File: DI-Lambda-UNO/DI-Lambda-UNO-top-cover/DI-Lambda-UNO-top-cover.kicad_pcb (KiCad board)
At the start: 2 copper layers, 38.2 x 68.5 mm, 7 parts, among them J12 Conn_01x05, J13 Conn_01x11, J5 Conn_01x11, SW2 SW_BLANK, SW3 SW_SAMPLE, SW4 SW_MODE, U1 LCD_1.44_ST7735

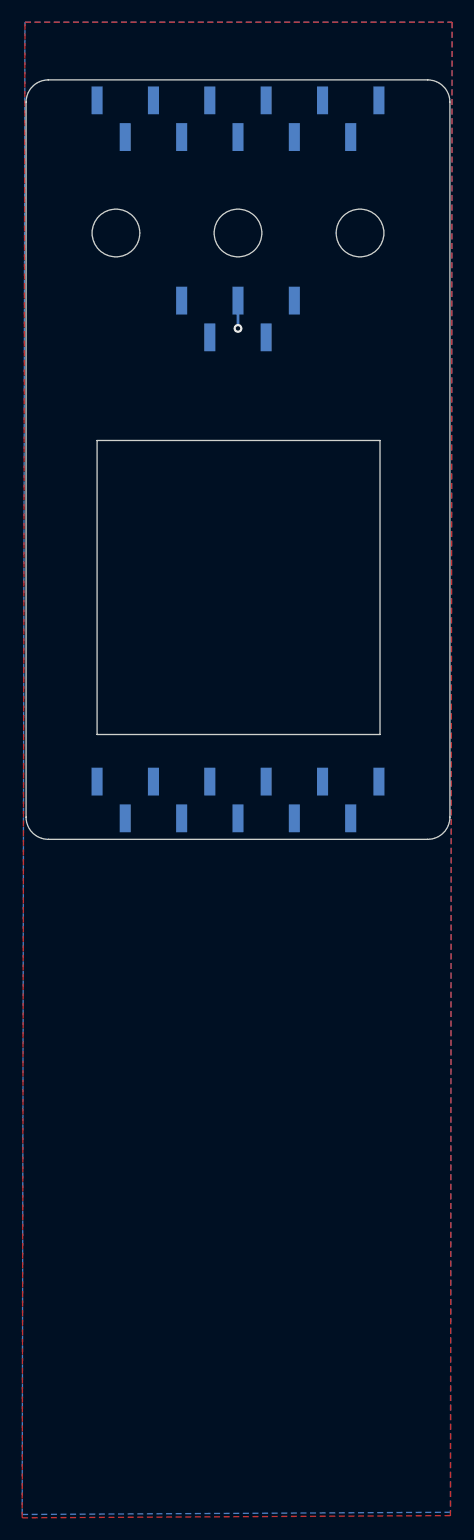
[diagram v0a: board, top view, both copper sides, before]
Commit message: Version 1.6
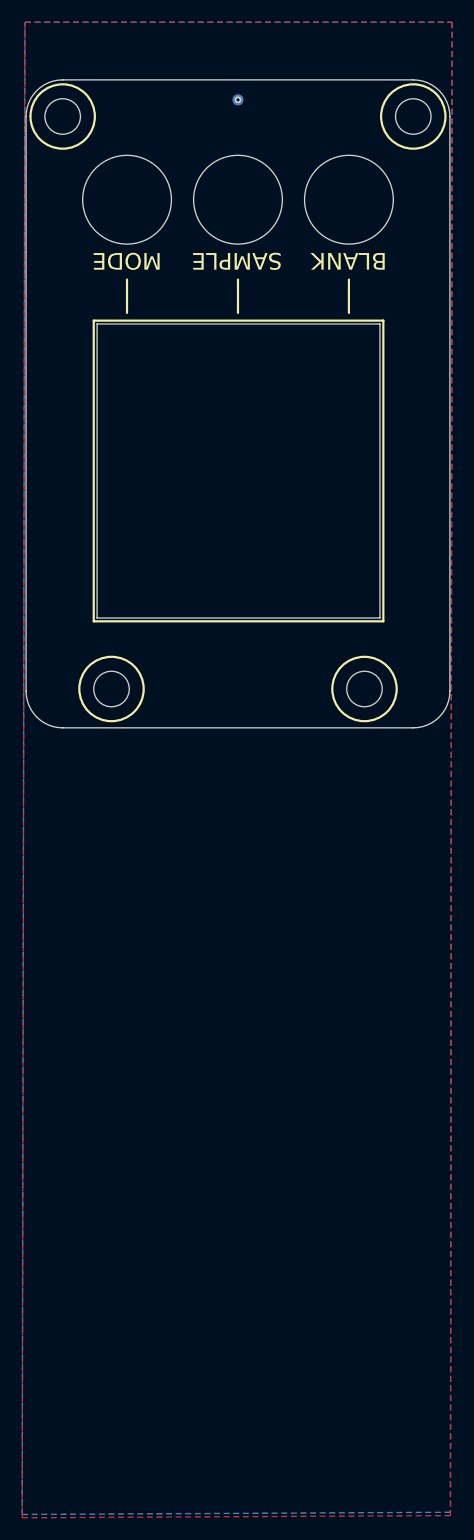
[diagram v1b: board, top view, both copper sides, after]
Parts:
- removed J12: Conn_01x05, Connector_PinHeader_2.54mm:PinHeader_1x05_P2.54mm_Vertical_SMD_Pin1Left
- removed J13, J5: Conn_01x11, Connector_PinHeader_2.54mm:PinHeader_1x11_P2.54mm_Vertical_SMD_Pin1Left
- added MK1: Mounting_Hole, MountingHole:MountingHole_3.2mm_M3, F.Cu at (134.6, 44.5)
- added MK2: Mounting_Hole, MountingHole:MountingHole_3.2mm_M3, F.Cu at (166.2, 44.5)
- added MK3: Mounting_Hole, MountingHole:MountingHole_3.2mm_M3, F.Cu at (139.0, 96.1)
- added MK4: Mounting_Hole, MountingHole:MountingHole_3.2mm_M3, F.Cu at (161.8, 96.1)
- added MK5: Mounting_Hole, DI-Lambda-module-tabs:Button_mounts_x3, F.Cu at (150.4, 44.5)
- added TP1: Test_Point, TestPoint:TestPoint_Pad_D1.0mm, B.Cu at (150.4, 43.0)
- SW2, SW3, SW4: footprint MountingHole:MountingHole_4.3mm_M4 -> DI-Lambda-module-tabs:Button-cutout
- moved U1 10.5 mm to (150.4, 64.1)
- moved SW3 3.16 mm to (160.4, 52.0), turned to 0 degrees
- moved SW4 3.16 mm to (140.4, 52.0), turned to 0 degrees
- moved SW2 3.00 mm to (150.4, 52.0), turned to 0 degrees
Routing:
- net GND: track 2.51 -> 0.00 mm
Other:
- board size 38.2 x 68.5 mm -> 38.2 x 58.4 mm
- net class Default: clearance 0.2 -> 0.15; trace_width 0.25 -> 0.15; via_dia 0.8 -> 0.6; via_drill 0.4 -> 0.3
- net class POWER added: clearance 0.2, trace_width 0.3, via_dia 0.6, via_drill 0.3
- rule pad_to_mask_clearance: 0.2 -> 0.07
- rule trace_clearance: 0.2 -> 0.15
- rule trace_min: 0.2 -> 0.15
- board text added: "BLANK"
- board text added: "DI-Lambda UNO v1.6"
- board text added: "MODE"
- board text added: "SAMPLE"
- board text removed: "Blank"
- board text removed: "DI-Lambda UNO v1.5"
- board text removed: "Mode"
- board text removed: "Sample"
